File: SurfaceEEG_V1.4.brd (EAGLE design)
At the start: 41.2 x 35.5 mm, 76 parts, among them IC1 LMV602, IC2 TSZ124IQ4T, U1 MCP4442-103E/ST, U2 ATMEGA328P-MU, U3 NRF24L01ALT1

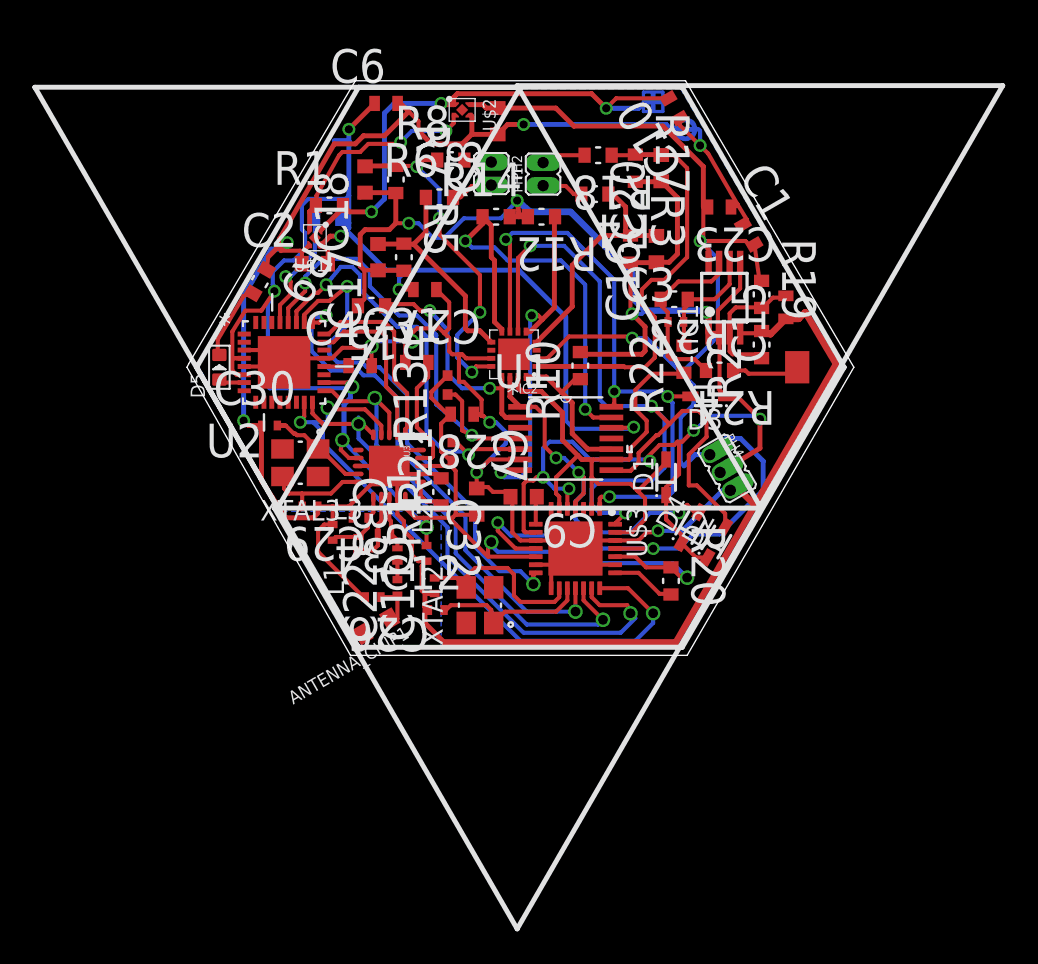
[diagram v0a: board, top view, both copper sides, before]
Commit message: Board changed after library changes
After making fonts smaller, the board have changed
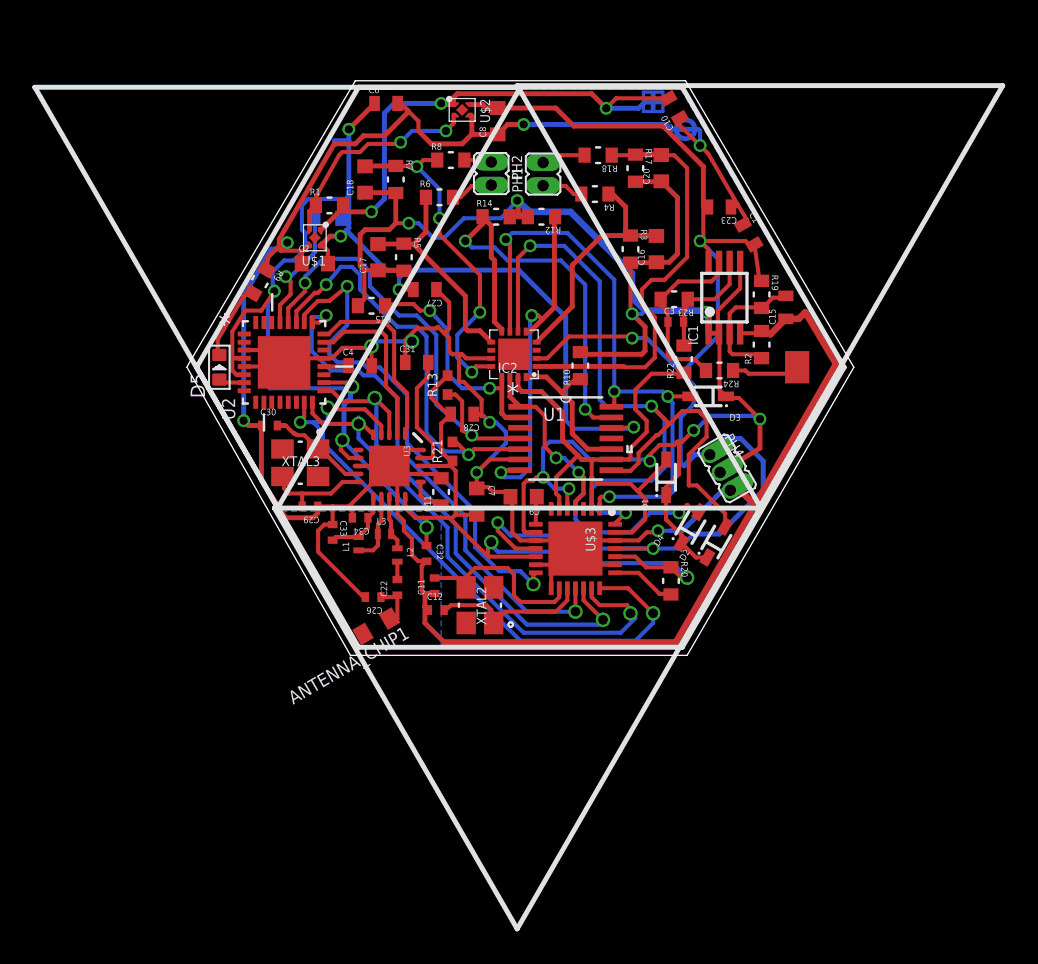
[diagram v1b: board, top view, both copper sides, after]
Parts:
- R19, R20: value 88.7K EDIT -> 82K Ohms
